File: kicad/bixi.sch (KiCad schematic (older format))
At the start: 35 parts, among them J1 RJ45, J10 Screw_Terminal_1x01, J2 RJ45, J3 RJ45, J4 RJ45, J5 RJ45, J6 RJ45, J7 RJ45, J8 RJ45, J9 Screw_Terminal_1x01, U1 Teensy3.6, U2 SP3485CN, U3 SP3485CN, U4 SP3485CN, U5 SP3485CN, U6 SP3485CN, U7 SP3485CN, U8 SP3485CN, U9 SP3485CN

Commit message: bixi node updates
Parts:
- removed J10, J9: Screw_Terminal_1x01, custom:A116169CT_SPADE_CONNECTOR, symbol Screw_Terminal_1x01
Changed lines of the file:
@@
 LIBS:valves
 LIBS:teensy
+LIBS:bixi-cache
 EELAYER 25 0
 EELAYER END
@@
 WS_8
 $Comp
-L GND #PWR057
-U 1 1 58BF15B9
-P 3750 6300
-F 0 "#PWR057" H 3750 6050 50  0001 C CNN
-F 1 "GND" H 3750 6150 50  0000 C CNN
-F 2 "" H 3750 6300 50  0000 C CNN
-F 3 "" H 3750 6300 50  0000 C CNN
-	1    3750 6300
-	1    0    0    -1
-$EndComp
-$Comp
-L VCC #PWR058
-U 1 1 58BF164F
-P 3750 5950
-F 0 "#PWR058" H 3750 5800 50  0001 C CNN
-F 1 "VCC" H 3750 6100 50  0000 C CNN
-F 2 "" H 3750 5950 50  0000 C CNN
-F 3 "" H 3750 5950 50  0000 C CNN
-	1    3750 5950
-	1    0    0    -1
-$EndComp
-$Comp
 L C C1
 U 1 1 58BF16CF
@@
 Connection ~ 6150 4300
 Connection ~ 6150 5550
-$Comp
-L Screw_Terminal_1x01 J9
-U 1 1 58EA496D
-P 3550 5950
-F 0 "J9" H 3550 6100 50  0000 C TNN
-F 1 "Screw_Terminal_1x01" V 3400 5950 50  0000 C TNN
-F 2 "custom:A116169CT_SPADE_CONNECTOR" H 3550 5825 50  0001 C CNN
-F 3 "" H 3550 5850 50  0001 C CNN
-	1    3550 5950
-	1    0    0    -1
-$EndComp
-$Comp
-L Screw_Terminal_1x01 J10
-U 1 1 58EA4A14
-P 3550 6300
-F 0 "J10" H 3550 6450 50  0000 C TNN
-F 1 "Screw_Terminal_1x01" V 3400 6300 50  0000 C TNN
-F 2 "custom:A116169CT_SPADE_CONNECTOR" H 3550 6175 50  0001 C CNN
-F 3 "" H 3550 6200 50  0001 C CNN
-	1    3550 6300
-	1    0    0    -1
-$EndComp
 $EndSCHEMATC

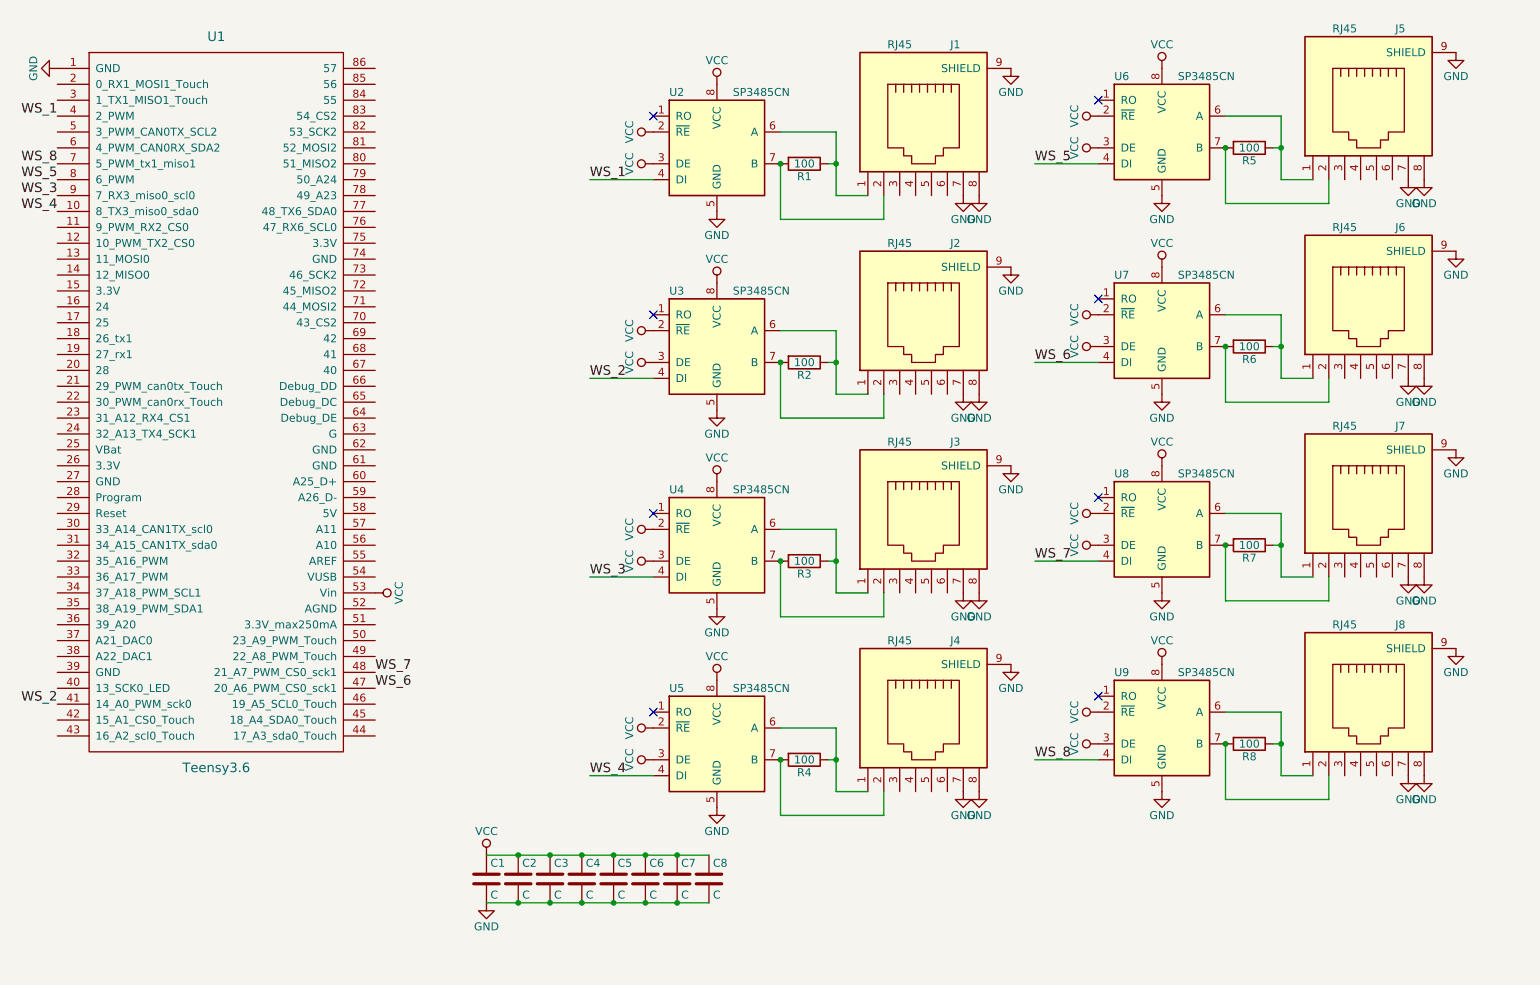
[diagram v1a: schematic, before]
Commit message: v3 pcb first pass
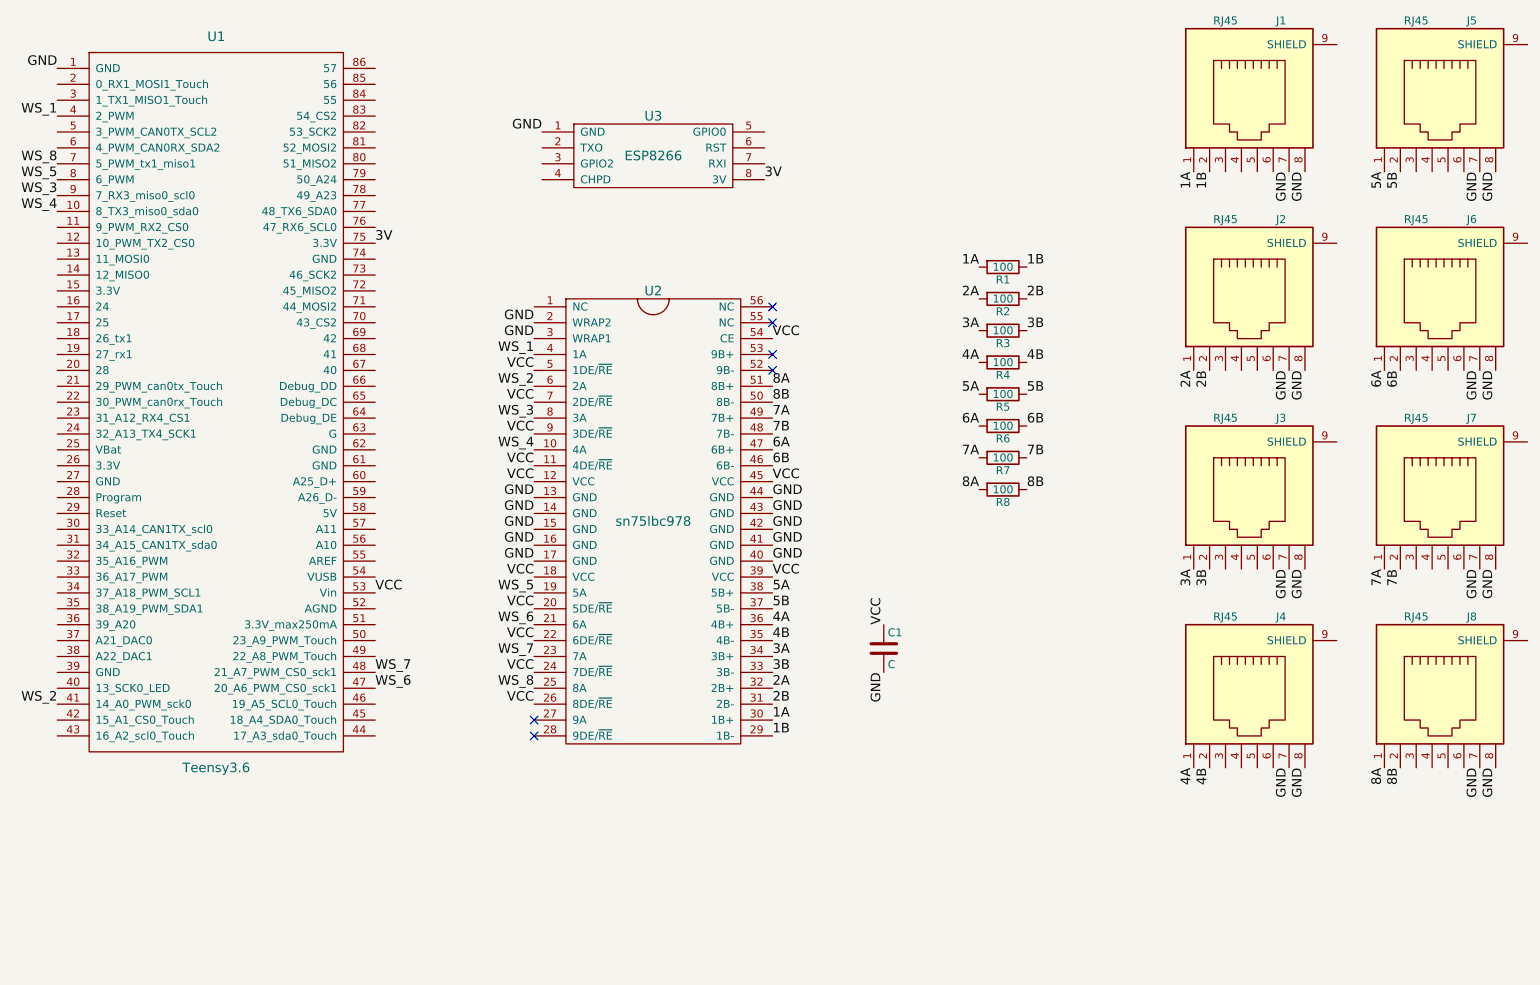
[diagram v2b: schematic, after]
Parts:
- removed C2, C3, C4, C5, C6, C7, C8: C, Capacitors_THT:C_Disc_D3_P2.5, symbol C
- removed U2, U3, U4, U5, U6, U7, U8, U9: SP3485CN, Housings_DIP:DIP-8_W7.62mm, symbol SP3485CN
- added U2: sn75lbc978, Housings_SSOP:SSOP-56_7.5x18.5mm_Pitch0.635mm, symbol sn75lbc978
- added U3: ESP8266, custom:ESP8266, symbol ESP8266
- C1: footprint Capacitors_THT:C_Disc_D3_P2.5 -> Capacitors_THT:C_Disc_D4.7mm_W2.5mm_P5.00mm
- R1, R2, R3, R4, R5, R6, R7, R8: footprint Resistors_THT:Resistor_Horizontal_RM7mm -> Resistors_THT:R_Axial_DIN0207_L6.3mm_D2.5mm_P7.62mm_Horizontal
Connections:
- net GND: now also U2.13 (GND), U2.14 (GND), U2.15 (GND), U2.16 (GND), U2.17 (GND), U2.2 (WRAP2), U2.3 (WRAP1), U2.40 (GND), U2.41 (GND), U2.42 (GND), U2.43 (GND), U2.44 (GND), U3.1 (GND); no longer J1.9 (SHIELD), J2.9 (SHIELD), J3.9 (SHIELD), J4.9 (SHIELD), J5.9 (SHIELD), J6.9 (SHIELD), J7.9 (SHIELD), J8.9 (SHIELD)
- net VCC: now also U2.11 (4DE/~RE), U2.12 (VCC), U2.18 (VCC), U2.20 (5DE/~RE), U2.22 (6DE/~RE), U2.24 (7DE/~RE), U2.26 (8DE/~RE), U2.39 (VCC), U2.45 (VCC), U2.5 (1DE/~RE), U2.54 (CE), U2.7 (2DE/~RE), U2.9 (3DE/~RE)
- net WS_1: now also U2.4 (1A)
- net WS_2: now also U2.6 (2A)
- net WS_3: now also U2.8 (3A)
- net WS_4: now also U2.10 (4A)
- net WS_5: now also U2.19 (5A)
- net WS_6: now also U2.21 (6A)
- net WS_7: now also U2.23 (7A)
- net WS_8: now also U2.25 (8A)
- net 8A: now reaches J8.1
- net 8A: now also R8.2, U2.51 (8B+); no longer R8.1
- net 8B: now reaches J8.2
- net 8B: now also R8.1, U2.50 (8B-); no longer R8.2
- net 3V: now reaches U1.75 (3.3V)
- net 3V: now also U3.8 (3V)
- net 7A: now reaches J7.1
- net 7A: now also R7.2, U2.49 (7B+); no longer R7.1
- net 7B: now reaches J7.2
- net 7B: now also R7.1, U2.48 (7B-); no longer R7.2
- net 6A: now reaches J6.1
- net 6A: now also R6.2, U2.47 (6B+); no longer R6.1
- net 6B: now reaches J6.2
- net 6B: now also R6.1, U2.46 (6B-); no longer R6.2
- net 5A: now reaches J5.1
- net 5A: now also R5.2, U2.38 (5B+); no longer R5.1
- net 5B: now reaches J5.2
- net 5B: now also R5.1, U2.37 (5B-); no longer R5.2
- net 4A: now reaches J4.1
- net 4A: now also R4.2, U2.36 (4B+); no longer R4.1
- net 4B: now reaches J4.2
- net 4B: now also R4.1, U2.35 (4B-); no longer R4.2
- net 3A: now reaches J3.1
- net 3A: now also R3.2, U2.34 (3B+); no longer R3.1
- net 3B: now reaches J3.2
- net 3B: now also R3.1, U2.33 (3B-); no longer R3.2
- net 2A: now reaches J2.1
- net 2A: now also R2.2, U2.32 (2B+); no longer R2.1
- net 2B: now reaches J2.2
- net 2B: now also R2.1, U2.31 (2B-); no longer R2.2
- net 1A: now reaches J1.1
- net 1A: now also R1.2, U2.30 (1B+); no longer R1.1
- net 1B: now reaches J1.2
- net 1B: now also R1.1, U2.29 (1B-); no longer R1.2
- no-connect marks 8 -> 6
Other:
- moved on the sheet: C1, J1, J2, J3, J4, J5, J6, J7, J8
